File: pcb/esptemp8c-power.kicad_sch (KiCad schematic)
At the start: 25 parts, among them J3 24VAC, J5 USB_C_Receptacle_USB2.0, U2 LMR54406DBVR

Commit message: docs and pics
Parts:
- D5: value CUS05S40.H3F -> 1N5819WS; LCSC C2762696 -> C191023
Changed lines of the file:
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@@
 			)
 		)
-		(property "Value" "CUS05S40.H3F"
+		(property "Value" "1N5819WS"
 			(at 125.984 97.79 0)
 			(effects
@@
 			)
 		)
-		(property "LCSC" "C2762696"
+		(property "LCSC" "C191023"
 			(at 125.73 101.6 0)
 			(effects

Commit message: fix footprint to sot23
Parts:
- U2: footprint Package_TO_SOT_SMD:TSOT-23-6 -> Package_TO_SOT_SMD:SOT-23-6
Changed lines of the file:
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@@
 			)
 		)
-		(property "Footprint" "Package_TO_SOT_SMD:TSOT-23-6"
+		(property "Footprint" "Package_TO_SOT_SMD:SOT-23-6"
 			(at 174.625 82.55 0)
 			(effects
@@
 			)
 		)
+		(property "Notes" ""
+			(at 173.99 76.2 0)
+			(effects
+				(font
+					(size 1.27 1.27)
+				)
+			)
+		)

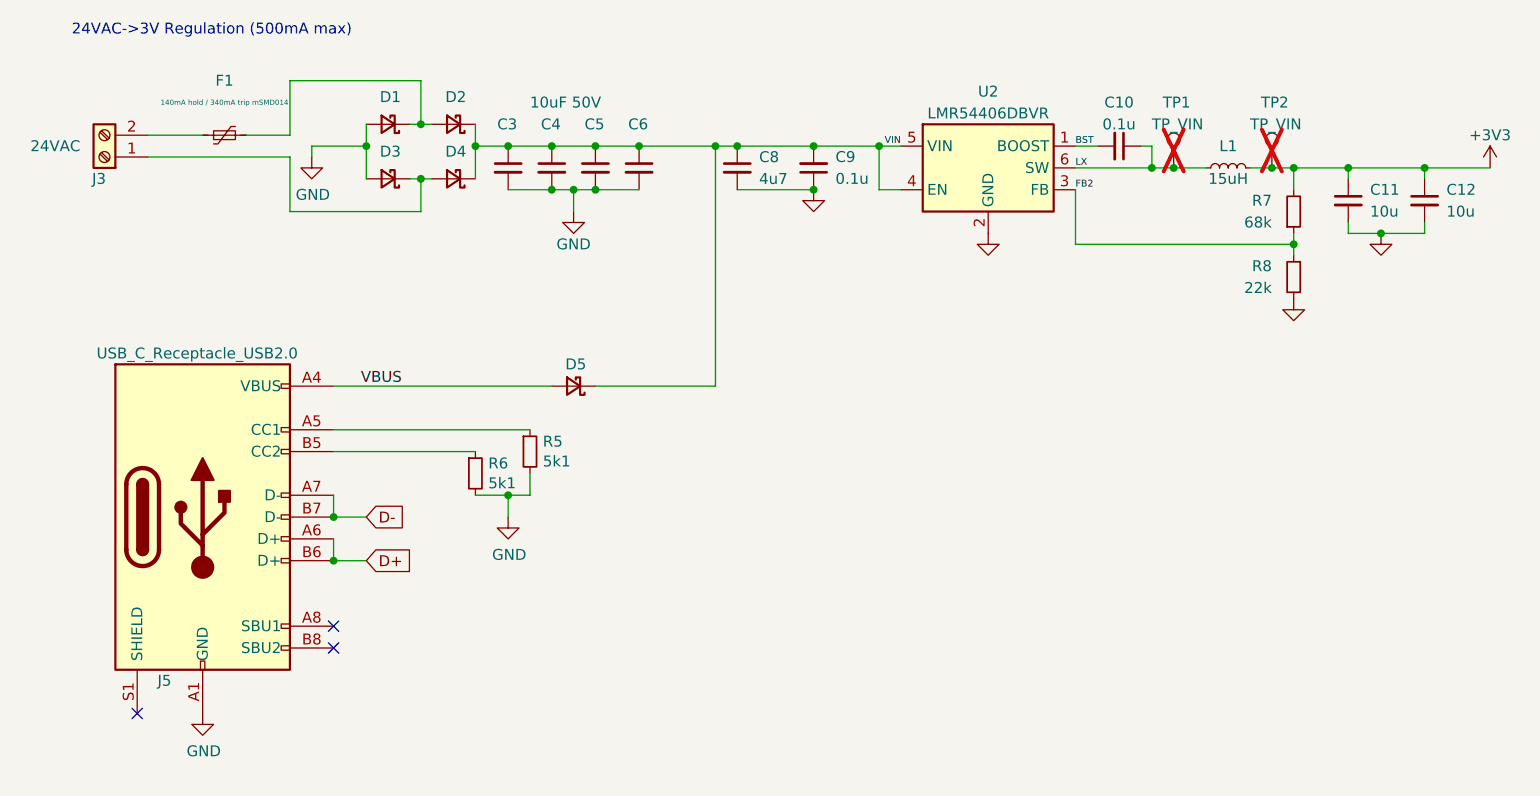
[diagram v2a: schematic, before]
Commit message: final touches and check
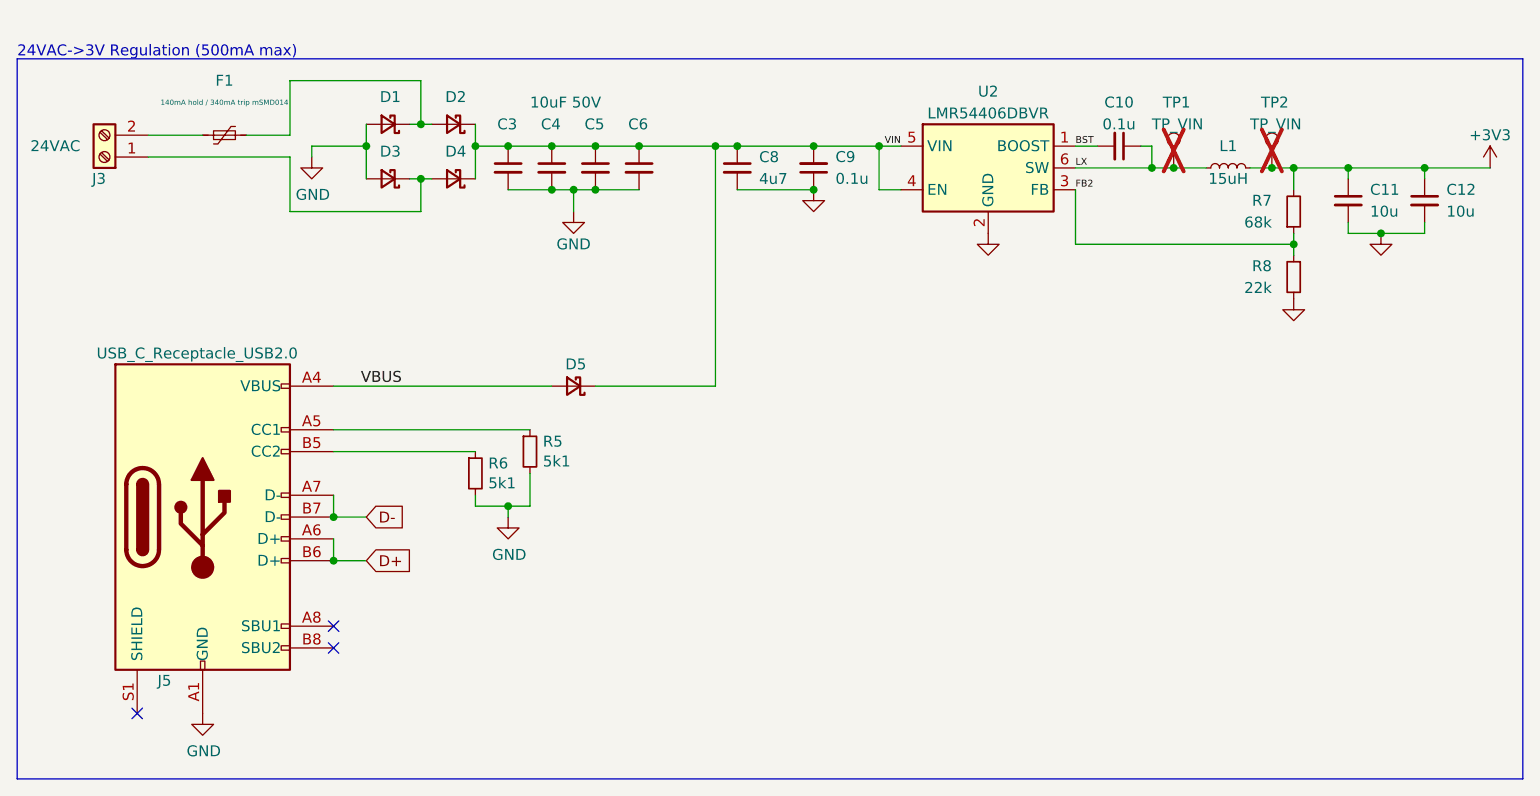
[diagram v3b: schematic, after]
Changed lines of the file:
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@@
+	)
+	(junction
+		(at 118.11 115.57)
+		(diameter 0)
+		(color 0 0 0 0)
 	)
 	(junction
@@
 	(junction
 		(at 219.71 83.82)
-		(diameter 0)
-		(color 0 0 0 0)
-	)
-	(junction
-		(at 118.11 114.3)
 		(diameter 0)
 		(color 0 0 0 0)
@@
 	(wire
 		(pts
-			(xy 118.11 114.3) (xy 118.11 116.84)
+			(xy 118.11 115.57) (xy 118.11 116.84)
 		)
 		(stroke
@@
 	(wire
 		(pts
-			(xy 120.65 114.3) (xy 120.65 111.76)
+			(xy 120.65 115.57) (xy 120.65 111.76)
 		)
 		(stroke
@@
 	(wire
 		(pts
-			(xy 114.3 114.3) (xy 118.11 114.3)
+			(xy 114.3 115.57) (xy 118.11 115.57)
 		)
 		(stroke
@@
 	(wire
 		(pts
+			(xy 118.11 115.57) (xy 120.65 115.57)
+		)
+		(stroke
+			(width 0)
+			(type default)
+		)
+	)
+	(wire
+		(pts
 			(xy 142.24 73.66) (xy 144.78 73.66)
 		)
@@
 	(wire
 		(pts
-			(xy 118.11 114.3) (xy 120.65 114.3)
-		)
-		(stroke
-			(width 0)
-			(type default)
-		)
-	)
-	(wire
-		(pts
 			(xy 215.9 83.82) (xy 219.71 83.82)
 		)
@@
 	(wire
 		(pts
+			(xy 114.3 115.57) (xy 114.3 114.3)
+		)
+		(stroke
+			(width 0)
+			(type default)
+		)
+	)
+	(wire
+		(pts
 			(xy 95.25 73.66) (xy 95.25 74.93)
 		)
@@
 			(width 0)
 			(type default)
+		)
+	)
+	(rectangle
+		(start 60.96 63.5)
+		(end 236.22 147.32)
+		(stroke
+			(width 0)
+			(type default)
+		)
+		(fill
+			(type none)
 		)
 	)
 	(text "24VAC->3V Regulation (500mA max)"
 		(exclude_from_sim no)
-		(at 67.31 60.96 0)
+		(at 60.96 63.5 0)
 		(effects
 			(font
